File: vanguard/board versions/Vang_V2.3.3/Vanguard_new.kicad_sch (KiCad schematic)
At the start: 94 parts, among them J1 USB_C_Receptacle_USB2.0_16P, J2 Micro_SD_Card_Det1, J3 Conn_02x03_Odd_Even, J4 Conn_01x03, J5 Conn_01x03, J6 Conn_01x03, J7 Conn_01x02_Pin, Q4 BSS138, U10 ATmega4809-A, U11 TPS82130SILR, U12 AP2112K-3.3, U3 ATSAMD11D14A-M, U4 BMP390L, U5 BD1020HFV-TR, U6 AT25DF641A-SH-T, U8 BNO055, U9 TPS61092, Y1 Crystal

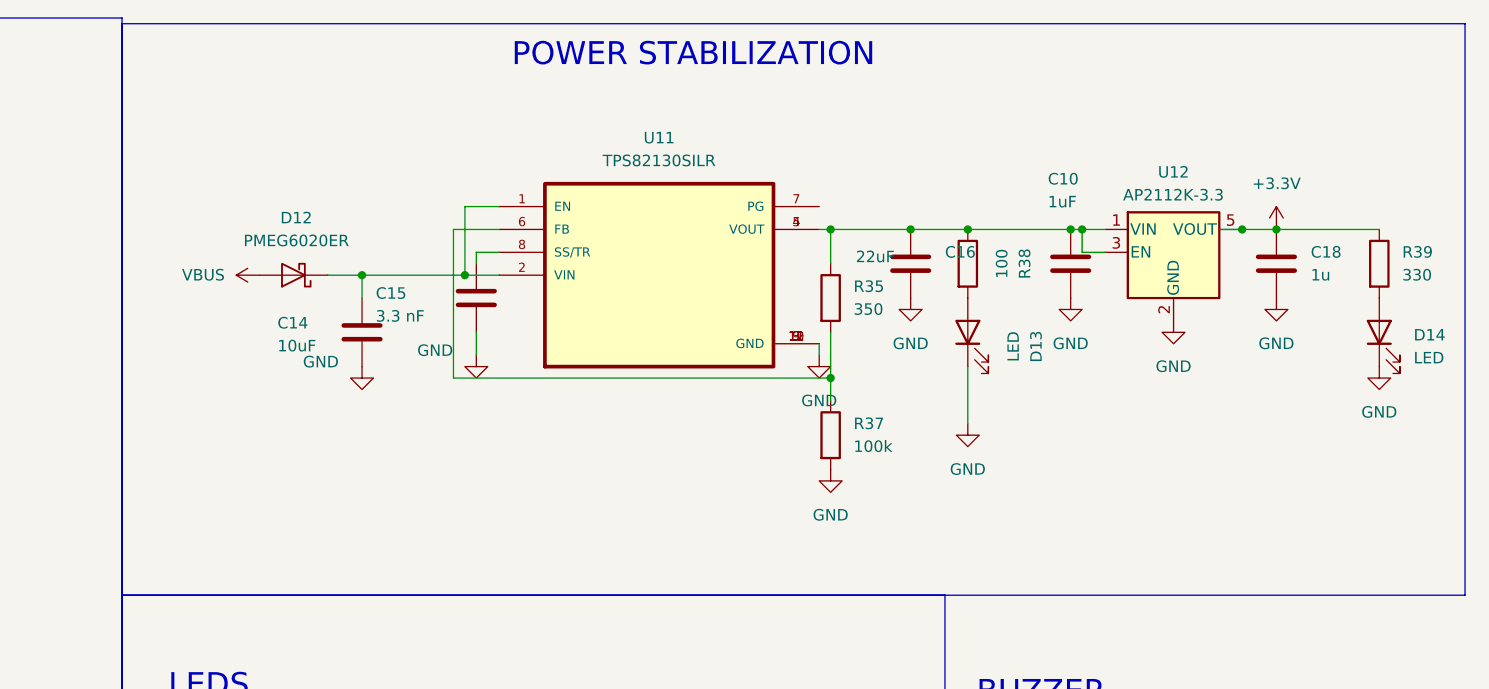
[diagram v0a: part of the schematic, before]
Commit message: finished input usb
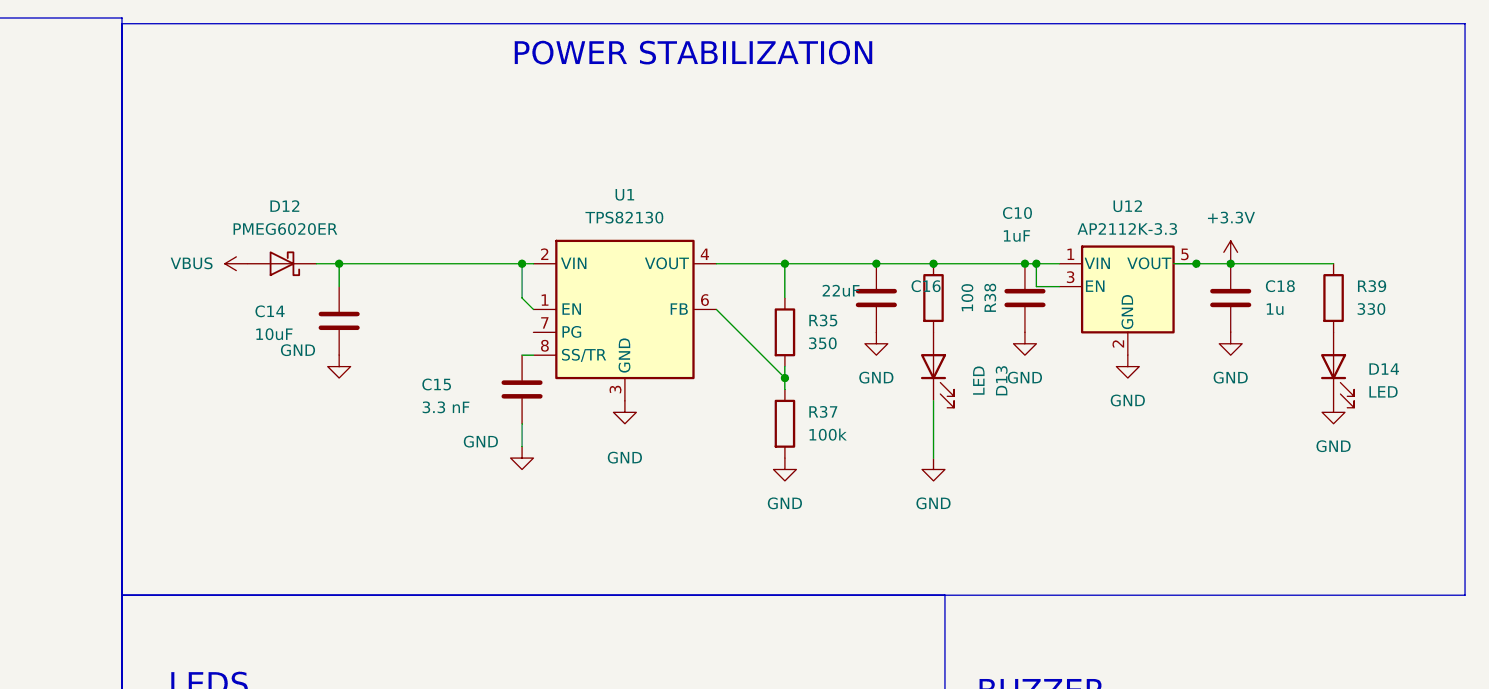
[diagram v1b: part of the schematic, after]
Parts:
- removed U11: TPS82130SILR, buck_convertor:CONV_TPS82140SILR.kicad_mod, symbol TPS82130SILR[1]:TPS82130SILR
- added U1: TPS82130, Package_LGA:Texas_SIL0008D_MicroSiP-8-1EP_2.8x3mm_P0.65mm_EP1.1x1.9mm_ThermalVias, symbol Regulator_Switching:TPS82130
- C1, C10, C11, C12, C14, C15, C16, C17, C18, C19, C2, C20, C21, C22, C3, C4, C5, C6, C7, C8: footprint Capacitor_SMD:C_0201_0603Metric -> Capacitor_SMD:C_0603_1608Metric
- C13: footprint Capacitor_SMD:CP_Elec_6.3x5.4 -> Capacitor_SMD:C_0603_1608Metric
- C26, C27: footprint (none) -> Capacitor_SMD:C_0603_1608Metric
- L1: footprint inductor:IND_SLF7055T-6R8N2R8-3PF.kicad_mod -> Package_LGA:ST_HLGA-10_2x2mm_P0.5mm_LayoutBorder3x2y
- R1, R10, R11, R12, R13, R2, R21, R22, R23, R24, R25, R26, R27, R28, R29, R3, R30, R31, R34, R35, R37, R38, R39, R4, R5, R6, R7, R8, R9: footprint Resistor_SMD:R_0402_1005Metric -> Resistor_SMD:R_0603_1608Metric
- R32, R33: footprint (none) -> Resistor_SMD:R_0603_1608Metric
- U4: footprint barometer:XDCR_BMP390L.kicad_mod -> Package_LGA:ST_HLGA-10_2x2mm_P0.5mm_LayoutBorder3x2y
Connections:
- net GND: now also U1.3 (GND), U1.9 (GND)
- net at C14.1, D12.1 (K): now also U1.1 (EN), U1.2 (VIN)
- net at C10.1, C16.1, R35.1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: now also U1.4 (VOUT), U1.5 (VOUT)
- net at R35.2, R37.1: now also U1.6 (FB)
- net at C15.1: now also U1.8 (SS/TR)
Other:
- moved on the sheet: C10, C14, C15, C16, C18, D12, D13, D14, R35, R37, R38, R39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
